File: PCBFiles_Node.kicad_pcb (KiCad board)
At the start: 2 copper layers, 68.5 x 29.9 mm, 33 parts, among them J1 Input, J2 Conn_01x04, J3 SPEC Sensor 968-001, J4 SHT31, J5 USB-TTL, J7 SMA, U1 STM32L431RCTx, U2 RFM9X, U3 STLQ015M33R, Y1 Q13FC1350000400 32.768kHz

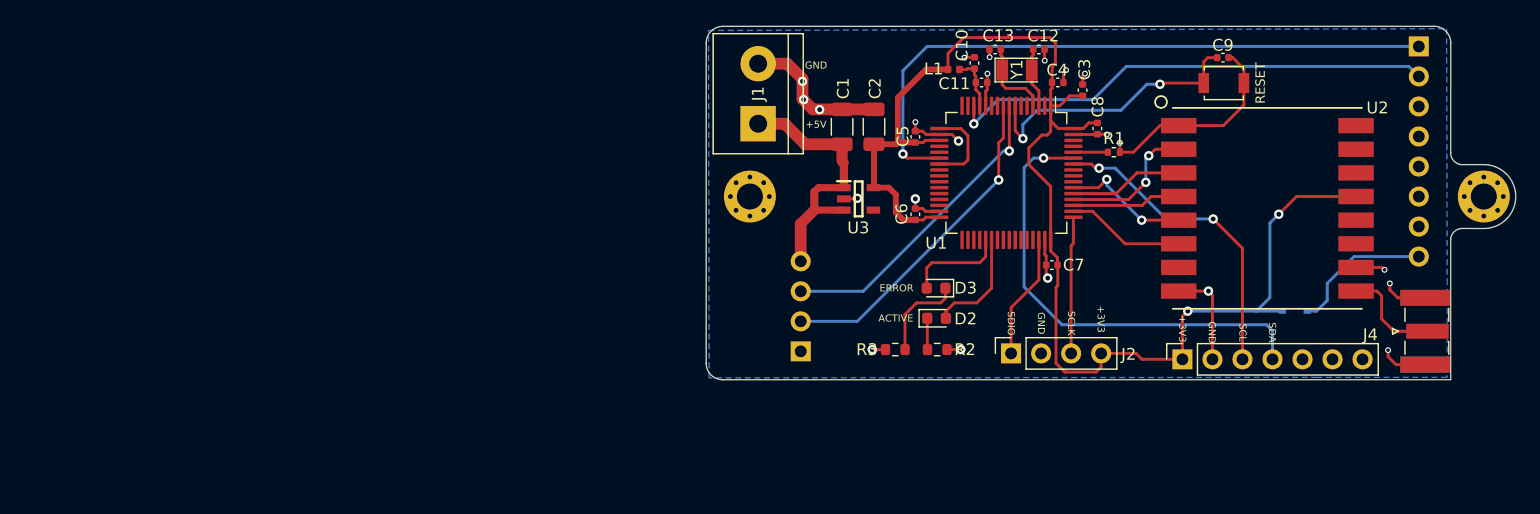
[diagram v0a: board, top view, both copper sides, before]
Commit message: Minor changes
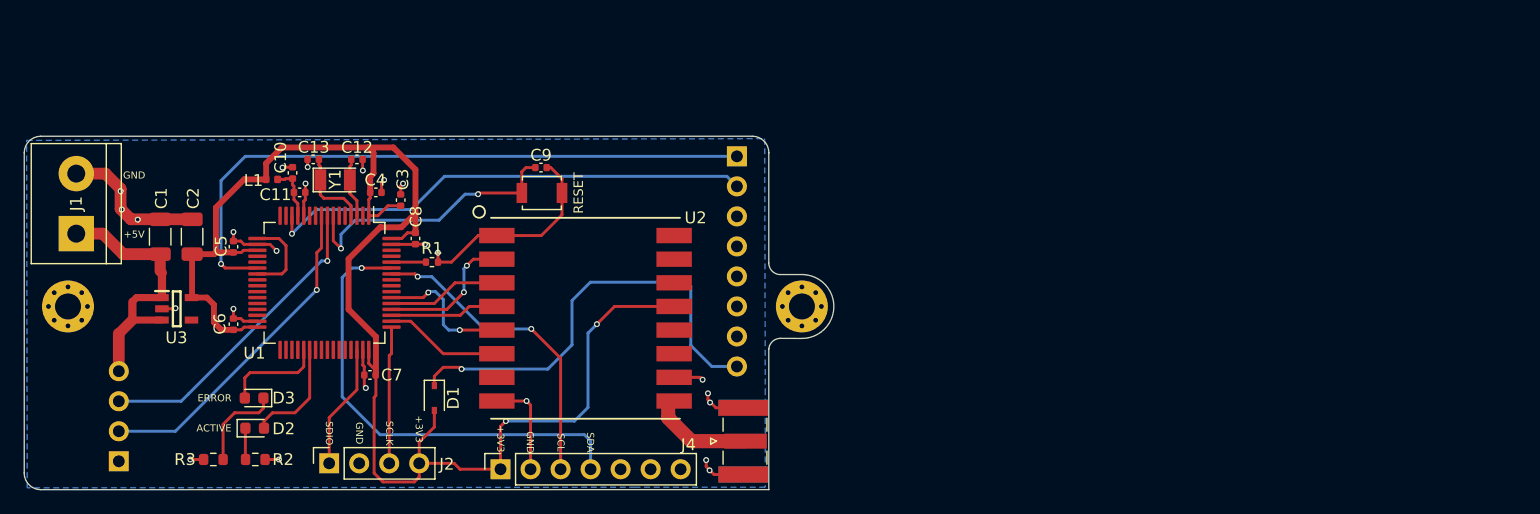
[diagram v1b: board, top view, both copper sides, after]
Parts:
- D1: moved to F.Cu
- moved D1 73.2 mm to (78.5, 106.0), turned to -90 degrees
- moved H1 58.4 mm to (109.6, 98.3)
- moved J3 58.4 mm to (104.1, 85.6)
- moved J4 58.4 mm to (84.1, 112.1)
- moved RESET 58.4 mm to (87.6, 88.7)
- moved U2 58.4 mm to (91.3, 99.3)
- moved C1 58.4 mm to (55.3, 92.4)
- moved C10 58.4 mm to (66.5, 87.0)
- moved C11 58.4 mm to (67.1, 88.7)
- moved C12 58.4 mm to (72.0, 85.9)
- moved C13 58.4 mm to (68.2, 85.9)
- moved C2 58.4 mm to (58.0, 92.4)
- moved C4 58.4 mm to (73.5, 88.7)
- moved C5 58.4 mm to (61.5, 93.2)
- moved C6 58.4 mm to (61.5, 99.8)
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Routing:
- net Net-(D1-Pad1): track 12.2 -> 37.9 mm, vias 0 -> 1
- net +3V3: track 114.5 -> 130.2 mm
- net SPI3_NSS: track 11.4 -> 12.2 mm
- net /ANT: track 9.54 -> 8.80 mm
- net GND: vias 22 -> 24
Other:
- board text added: "0.2000 mm / 0.0000 mm"
- board text added: "0.3000 mm"
- board text added: "1.6000 mm"
- board text added: "2"
- board text added: "68.6079 mm x 30.0066 mm"
- board text added: "BOARD CHARACTERISTICS"
- board text added: "Board Thickness:"
- board text added: "Board overall dimensions:"
- board text added: "Castellated pads:"
- board text added: "Copper Finish:"
- board text added: "Copper Layer Count:"
- board text added: "Edge card connectors:"
- board text added: "Impedance Control:"
- board text added: "Min hole diameter:"
- board text added: "Min track/spacing:"
- board text added: "No"
- board text added: "None"
- board text added: "Plated Board Edge:"
